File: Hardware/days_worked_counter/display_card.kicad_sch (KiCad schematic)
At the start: 39 parts, among them J501 Top Conn, J502 Bottom Conn, Q501 MMBT3904, Q502 MMBT3904, Q503 MMBT3904, Q504 MMBT3904, Q505 MMBT3906, Q506 MMBT3906, Q507 MMBT3906, Q508 MMBT3904, Q509 MMBT3906, Q510 MMBT3904, Q511 MMBT3904, Q513 MMBT3906, Q514 MMBT3906, Q515 MMBT3906, U501 SN74HC595

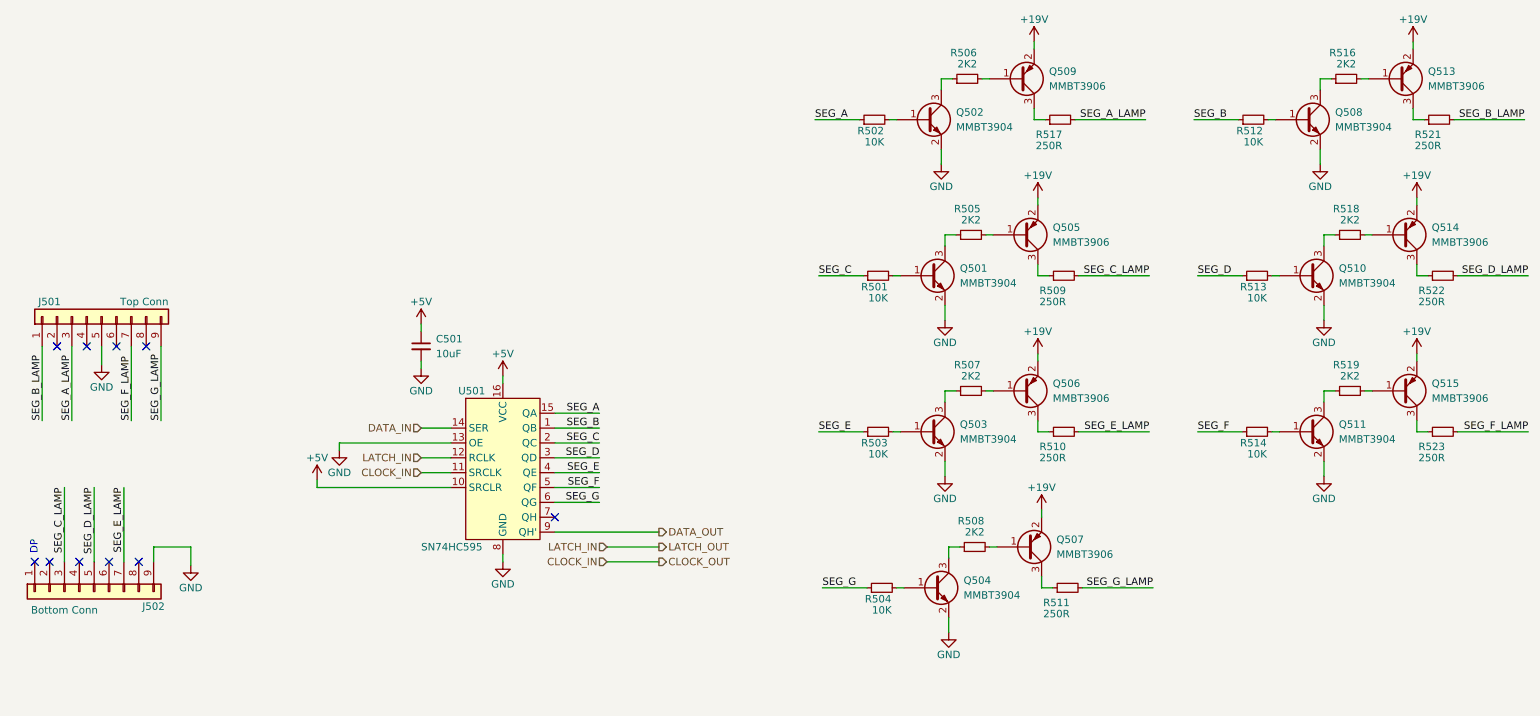
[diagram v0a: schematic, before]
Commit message: Change direction
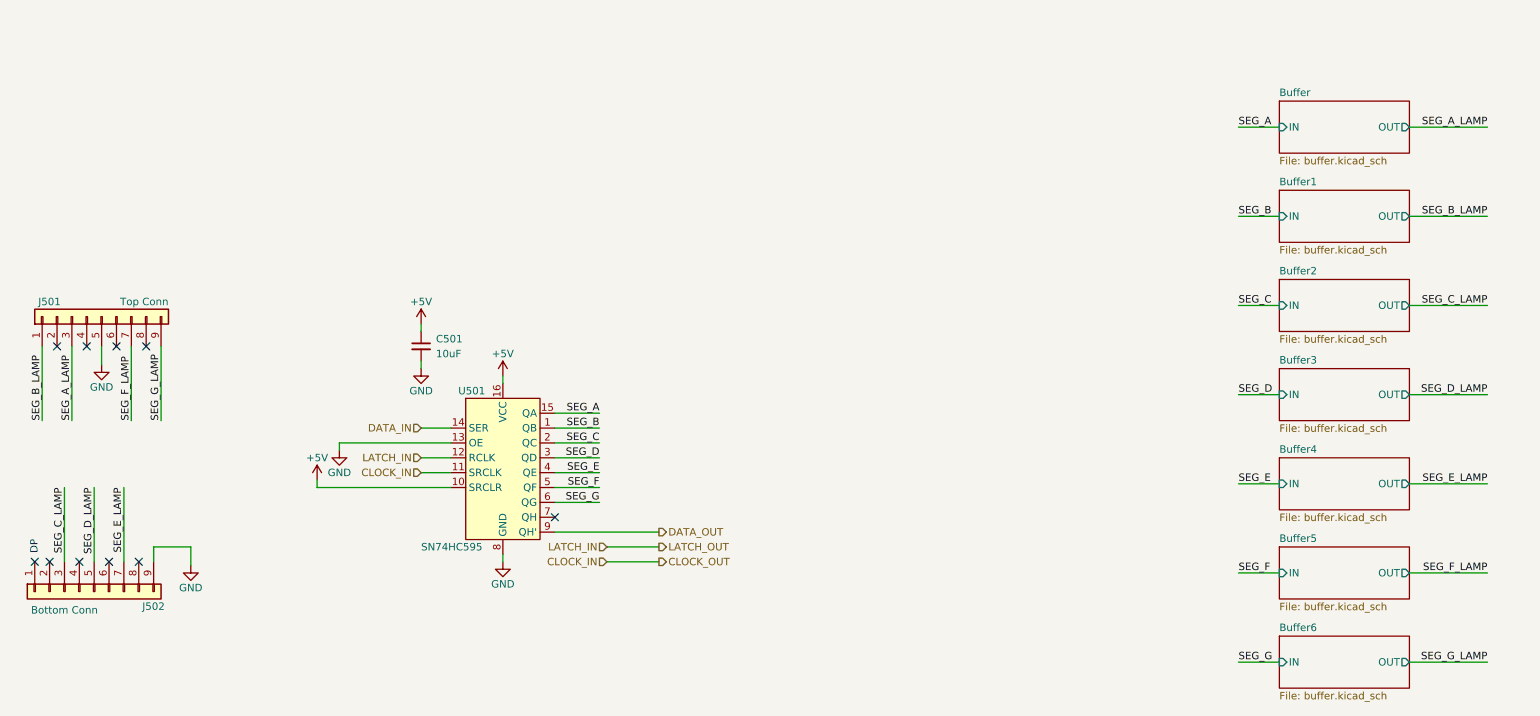
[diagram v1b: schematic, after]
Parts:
- removed Q501, Q502, Q503, Q504, Q508, Q510, Q511: MMBT3904, Package_TO_SOT_SMD:SOT-23, symbol Transistor_BJT:MMBT3904
- removed Q505, Q506, Q507, Q509, Q513, Q514, Q515: MMBT3906, Package_TO_SOT_SMD:SOT-23, symbol Transistor_BJT:MMBT3906
- removed R501, R502, R503, R504, R512, R513, R514: 10K, Resistor_SMD:R_0805_2012Metric, symbol Device:R_Small
- removed R505, R506, R507, R508, R516, R518, R519: 2K2, Resistor_SMD:R_0805_2012Metric, symbol Device:R_Small
- removed R509, R510, R511, R517, R521, R522, R523: 250R, Resistor_SMD:R_0805_2012Metric, symbol Device:R_Small
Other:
- added sheet Buffer (buffer.kicad_sch)
- added sheet Buffer1 (buffer.kicad_sch)
- added sheet Buffer2 (buffer.kicad_sch)
- added sheet Buffer3 (buffer.kicad_sch)
- added sheet Buffer4 (buffer.kicad_sch)
- added sheet Buffer5 (buffer.kicad_sch)
- added sheet Buffer6 (buffer.kicad_sch)
